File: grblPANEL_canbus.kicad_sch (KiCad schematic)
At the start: 14 parts, among them J301 Conn_01x02, U301 SN65HVD230

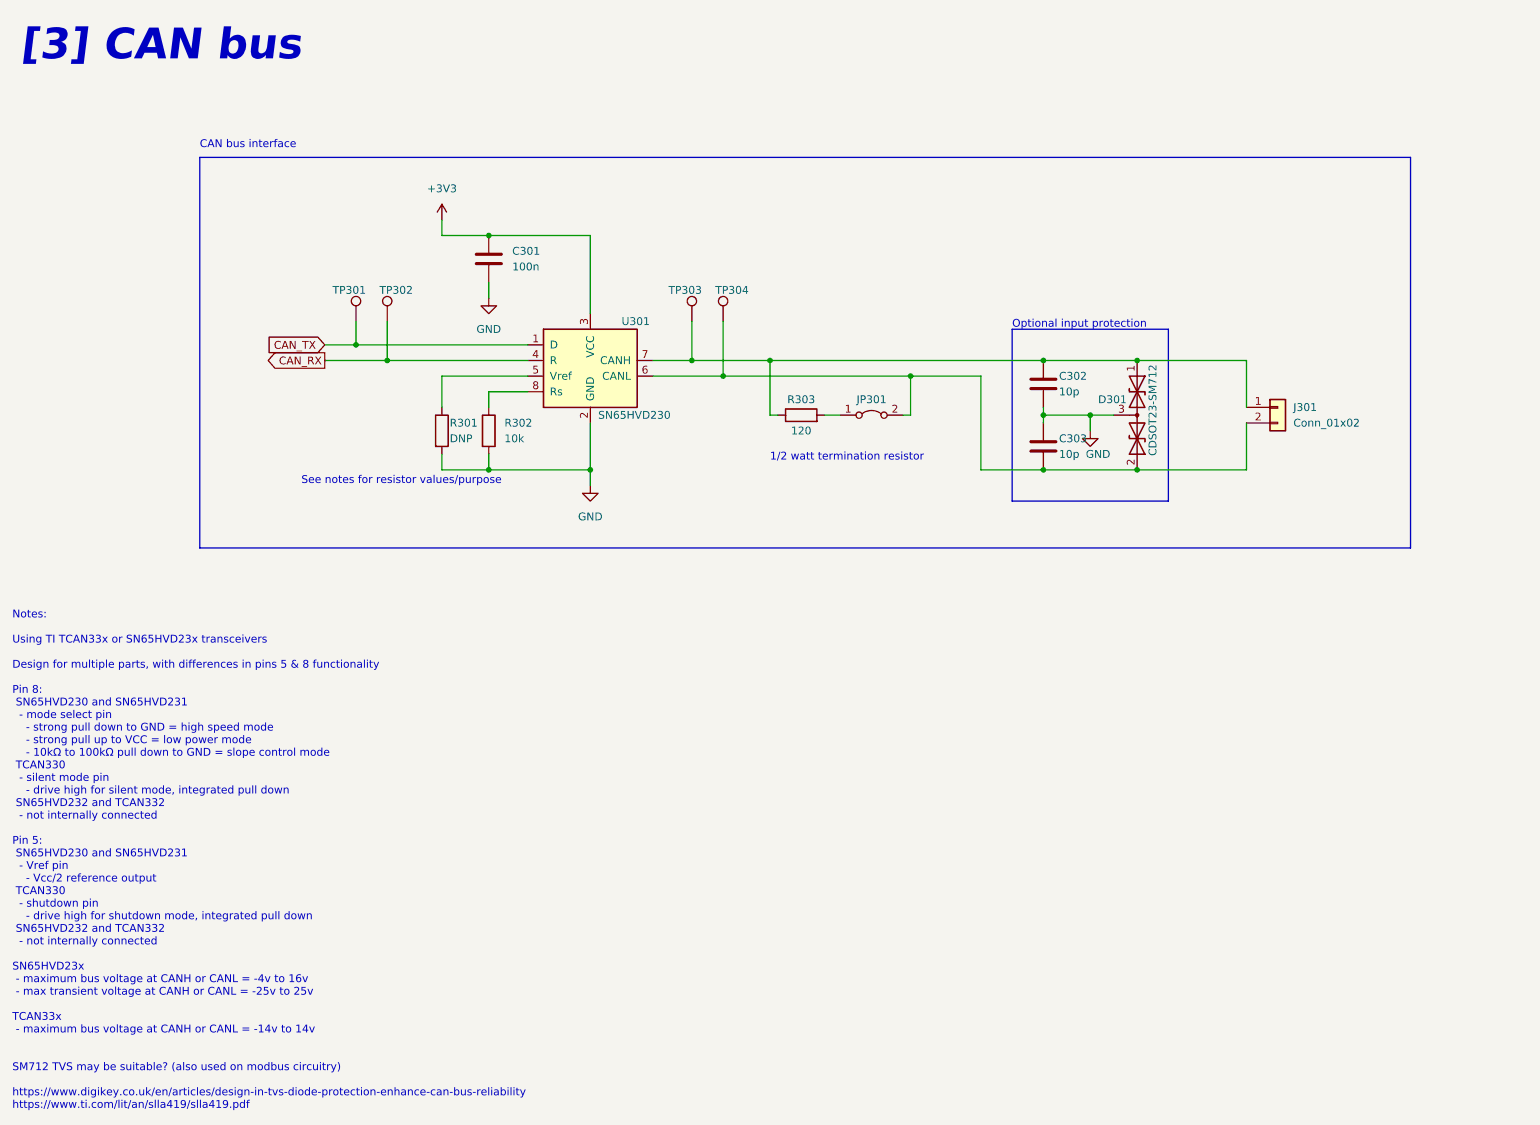
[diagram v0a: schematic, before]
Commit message: Refresh
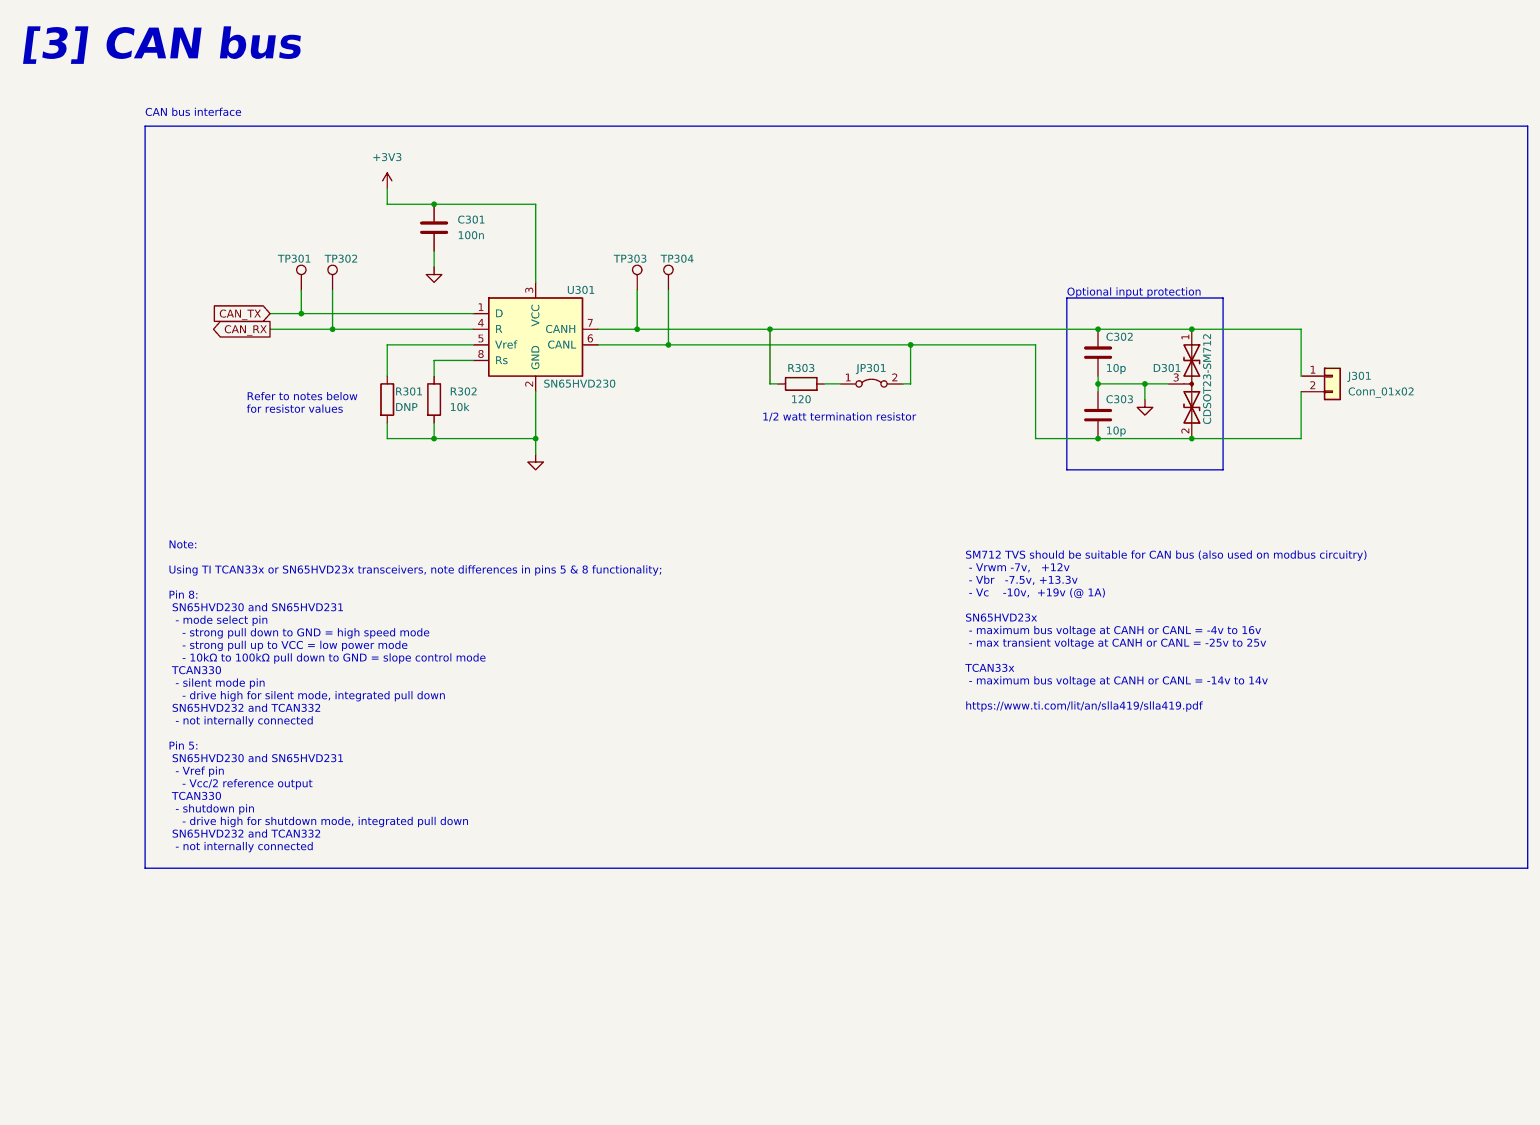
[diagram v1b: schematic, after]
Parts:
- C301, C302, C303: footprint (none) -> Capacitor_SMD:C_0603_1608Metric
- D301: footprint (none) -> Package_TO_SOT_SMD:SOT-23
- J301: footprint (none) -> TerminalBlock_4Ucon:TerminalBlock_4Ucon_1x02_P3.50mm_Horizontal
- JP301: footprint (none) -> Connector_Pin:Pin_D1.1mm_L8.5mm_W2.5mm_FlatFork
- R301, R302, R303: footprint (none) -> Resistor_SMD:R_0603_1608Metric
- TP301, TP302, TP303, TP304: footprint (none) -> Connector_Pin:Pin_D1.0mm_L10.0mm
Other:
- note added: "Note: Using TI TCAN33x or SN65HVD23x transceivers, note differences in pins 5 & 8 functionality; Pin 8: SN65HVD230 and SN65HVD231 - mode select pin - strong pull down to GND = high speed mode - strong pull up to VCC = low power mode - 10kΩ to 100kΩ pull down to GND = slope control mode TCAN330 - silent mode pin - drive high for silent mode, integrated pull down SN65HVD232 and TCAN332 - not intern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"
- note added: "Refer to notes below for resistor values"
- note added: "SM712 TVS should be suitable for CAN bus (also used on modbus circuitry) - Vrwm -7v, +12v - Vbr -7.5v, +13.3v - Vc -10v, +19v (@ 1A) SN65HVD23x - maximum bus voltage at CANH or CANL = -4v to 16v - max transient voltage at CANH or CANL = -25v to 25v TCAN33x - maximum bus voltage at CANH or CANL = -14v to 14v https://www.ti.com/lit/an/slla419/slla419.pdf"
- note removed: "Notes: Using TI TCAN33x or SN65HVD23x transceivers Design for multiple parts, with differences in pins 5 & 8 functionality Pin 8: SN65HVD230 and SN65HVD231 - mode select pin - strong pull down to GND = high speed mode - strong pull up to VCC = low power mode - 10kΩ to 100kΩ pull down to GND = slope control mode TCAN330 - silent mode pin - drive high for silent mode, integrated pull down SN65HVD23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"
- note removed: "See notes for resistor values/purpose"
- moved on the sheet: C301, C302, C303, D301, J301, JP301, R301, R302, R303, TP301, TP302, TP303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
